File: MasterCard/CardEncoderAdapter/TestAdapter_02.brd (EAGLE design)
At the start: 64.5 x 31.1 mm, 35 parts, among them IC1 STM32F103T4U6A, IC2 LD1117STR, IC3 MAX3232CUE, J1 POWER_JACK, Q1 12MHz, SW2 BUTTON6X3.5, X1 USB-MINIMICROMICRO

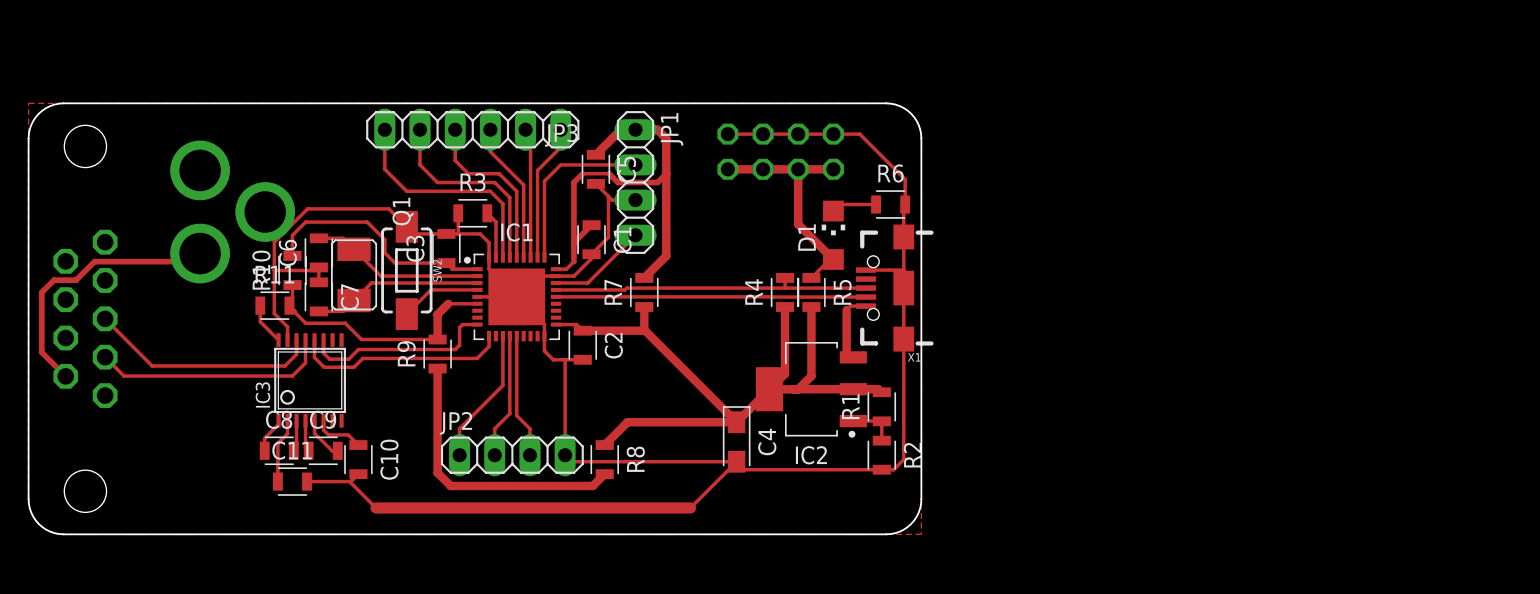
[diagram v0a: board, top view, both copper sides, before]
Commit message: _
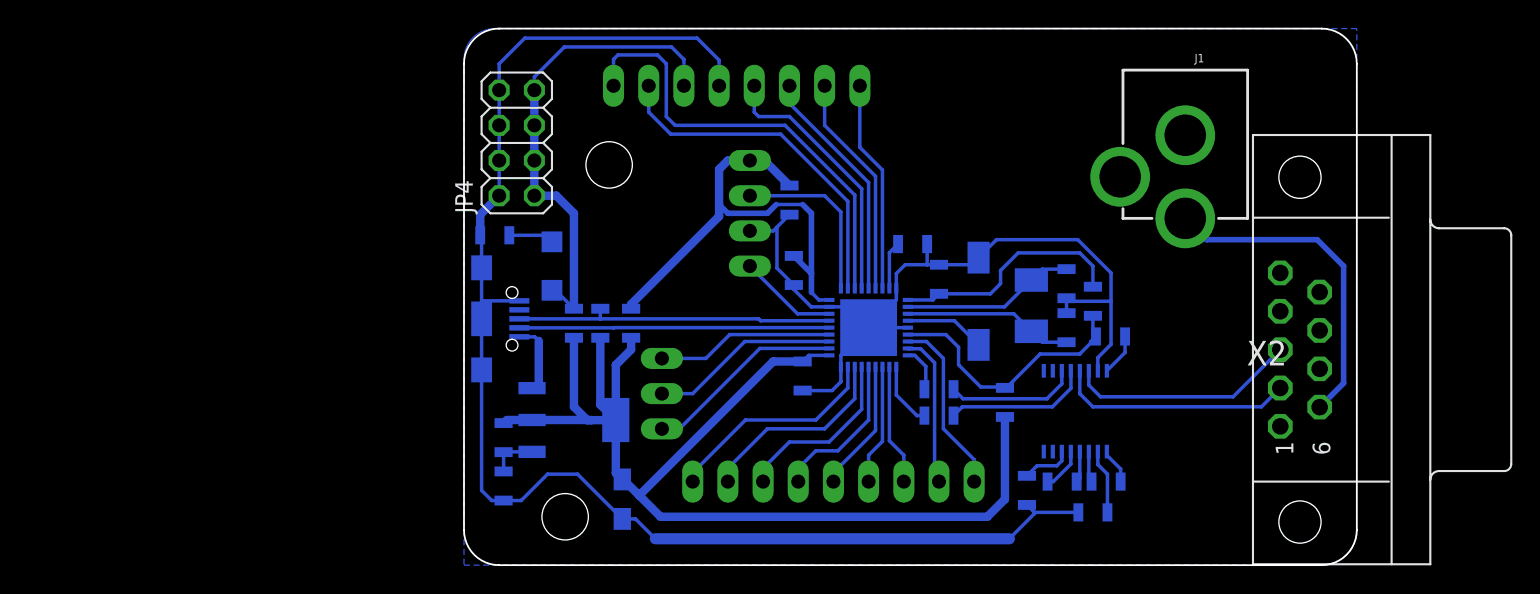
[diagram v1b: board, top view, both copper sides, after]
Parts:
- removed R8: 0, Flamberm:RESC2012X50
- added JP5: (no value), pinhead:1X08
- added R12, R13: 0, Flamberm:RESC2012X50
- JP2: device pinhead:1X04 -> pinhead:1X09
- JP3: device pinhead:1X06 -> pinhead:1X03
- moved X2 106.7 mm to (69.8, 15.6), flipped to the top
- moved J1 71.2 mm to (52.1, 38.7), flipped to the top
- moved R11 60.4 mm to (46.7, 16.5), flipped to the bottom
- moved C8 59.7 mm to (46.4, 6.03), flipped to the bottom
- moved C11 57.8 mm to (45.4, 3.81), flipped to the bottom
- moved R10 57.8 mm to (45.4, 19.1), flipped to the bottom
- moved IC3 55.3 mm to (44.1, 11.1), flipped to the bottom
- moved C6 54.0 mm to (43.5, 20.3), flipped to the bottom
- moved C7 54.0 mm to (43.5, 17.1), flipped to the bottom
- moved C9 53.4 mm to (43.2, 6.03), flipped to the bottom
- moved Q1 48.9 mm to (41.0, 18.7), flipped to the bottom
- moved C10 48.3 mm to (40.6, 5.40), flipped to the bottom
- moved SW2 41.3 mm to (37.1, 19.1), flipped to the bottom
- moved R9 41.1 mm to (39.1, 11.7), flipped to the bottom
- moved C3 35.6 mm to (34.3, 20.6), flipped to the bottom
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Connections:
- removed net DISP_D4: IC1.31, JP3.3
- removed net DISP_D5: IC1.32, JP3.4
- removed net DISP_D6: IC1.33, JP3.5
- removed net DISP_D7: IC1.34, JP3.6
- removed net DISP_DC: IC1.30, JP3.2
- removed net DISP_E: IC1.29, JP3.1
- removed net N$7: R8.2, R9.1
- removed net SPI1_MISO: IC1.13, JP2.2
- removed net SPI1_MOSI: IC1.14, JP2.3
- removed net SPI1_SCK: IC1.12, JP2.1
- new net N$8: IC1.10, R12.1
- new net N$9: IC1.9, R13.1
- new net PA0: IC1.7, JP2.1
- new net PA1: IC1.8, JP2.2
- new net PA10: IC1.22, JP3.3
- new net PA15_DISP_E: IC1.29, JP5.2
- new net PA4: IC1.11, JP2.3
- new net PA5_SPI1_SCK: IC1.12, JP2.4
- new net PA6_SPI1_MISO: IC1.13, JP2.5
- new net PA7_SPI1_MOSI: IC1.14, JP2.6
- new net PA8: IC1.20, JP3.1
- new net PA9: IC1.21, JP3.2
- new net PB0: IC1.15, JP2.7
- new net PB1: IC1.16, JP2.8
- new net PB2: IC1.17, JP2.9
- new net PB3_DISP_DC: IC1.30, JP5.1
- new net PB4_DISP_D4: IC1.31, JP5.5
- new net PB5_DISP_D5: IC1.32, JP5.6
- new net PB6_DISP_D6: IC1.33, JP5.7
- new net PB7_DISP_D7: IC1.34, JP5.8
- net +3V3: now also R9.1; no longer R8.1
- net GND: now also JP5.4; no longer JP2.4
- net N$16: now also R13.2; no longer IC1.9
- net N$17: now also R12.2; no longer IC1.10
- net N$25: now also JP5.3
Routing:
- net +3V3: track 52.5 -> 85.3 mm
- net PB3_DISP_DC: track 0.00 -> 32.6 mm
- net PA15_DISP_E: track 0.00 -> 25.2 mm
- net N$7: track 20.3 -> 0.00 mm
- net PB4_DISP_D4: track 0.00 -> 19.1 mm
- net N$25: track 17.3 -> 35.0 mm
- net PB5_DISP_D5: track 0.00 -> 17.0 mm
- net DISP_D7: track 16.3 -> 0.00 mm
- net PB6_DISP_D6: track 0.00 -> 16.1 mm
- net PB2: track 0.00 -> 15.9 mm
- net PB7_DISP_D7: track 0.00 -> 15.3 mm
- net PA8: track 0.00 -> 14.5 mm
- net PB1: track 0.00 -> 14.5 mm
- net DISP_D6: track 14.3 -> 0.00 mm
- net PA9: track 0.00 -> 13.6 mm
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- added copper zone on layer 16, net GND
- removed copper zone on layer 1, net GND
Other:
- board size 64.5 x 31.1 mm -> 64.5 x 38.7 mm
